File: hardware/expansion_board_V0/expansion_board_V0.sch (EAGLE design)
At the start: 502 parts, among them CON1 ELEC, CON10 M5, CON11 M2, CON12 M4, CON13 M1, CON14 ESC0, CON15 CON10_2_2.54, CON16 CON10_2_2.54, CON17 ESC1, CON18 UART0, CON19 QEI1, CON2 SERVO, CON20 AN0, CON21 S0, CON22 IO0, CON23 AN1, CON24 S1, CON25 IO1, CON26 UART1, CON27 QEI0, CON28 AN2, CON29 S2, CON3 LIPO_MOT, CON30 IO2, CON31 TELEM, CON32 QEI3, CON33 AN3, CON34 S3, CON35 IO3, CON36 BALISE, CON37 AN4, CON38 S4, CON39 IO4, CON4 LIPO_MOT, CON40 SPI0, CON41 QEI2, CON42 AN5, CON43 S5, CON44 IO5, CON45 SPI1, CON46 AN6, CON47 S6, CON48 IO6, CON49 I2C0, CON5 LIPO_MOT, CON50 AN7, CON51 S7, CON52 IO7, CON53 I2C1, CON54 USB2, CON55 USB3, CON56 USBfpga, CON57 FPGA_GPIO0, CON58 FPGA_GPIO1, CON59 FPGA_LTC, CON6 LIPO_MOT, CON60 USB3, CON61 CON5_2.54S, CON62 CON5_2.54S, CON63 CON5_2.54S, CON64 CON5_2.54S, CON7 FPGApower, CON8 M0, CON9 M3, IC1 ADS1258, IC2 ADS1278, IC3 REF5030I, IC4 REF5025I, J1 NC, J10 0, J11 0, J12 0, J13 0, J14 0, J15 0, J16 0, J17 0, J18 0, J19 0, J2 nc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

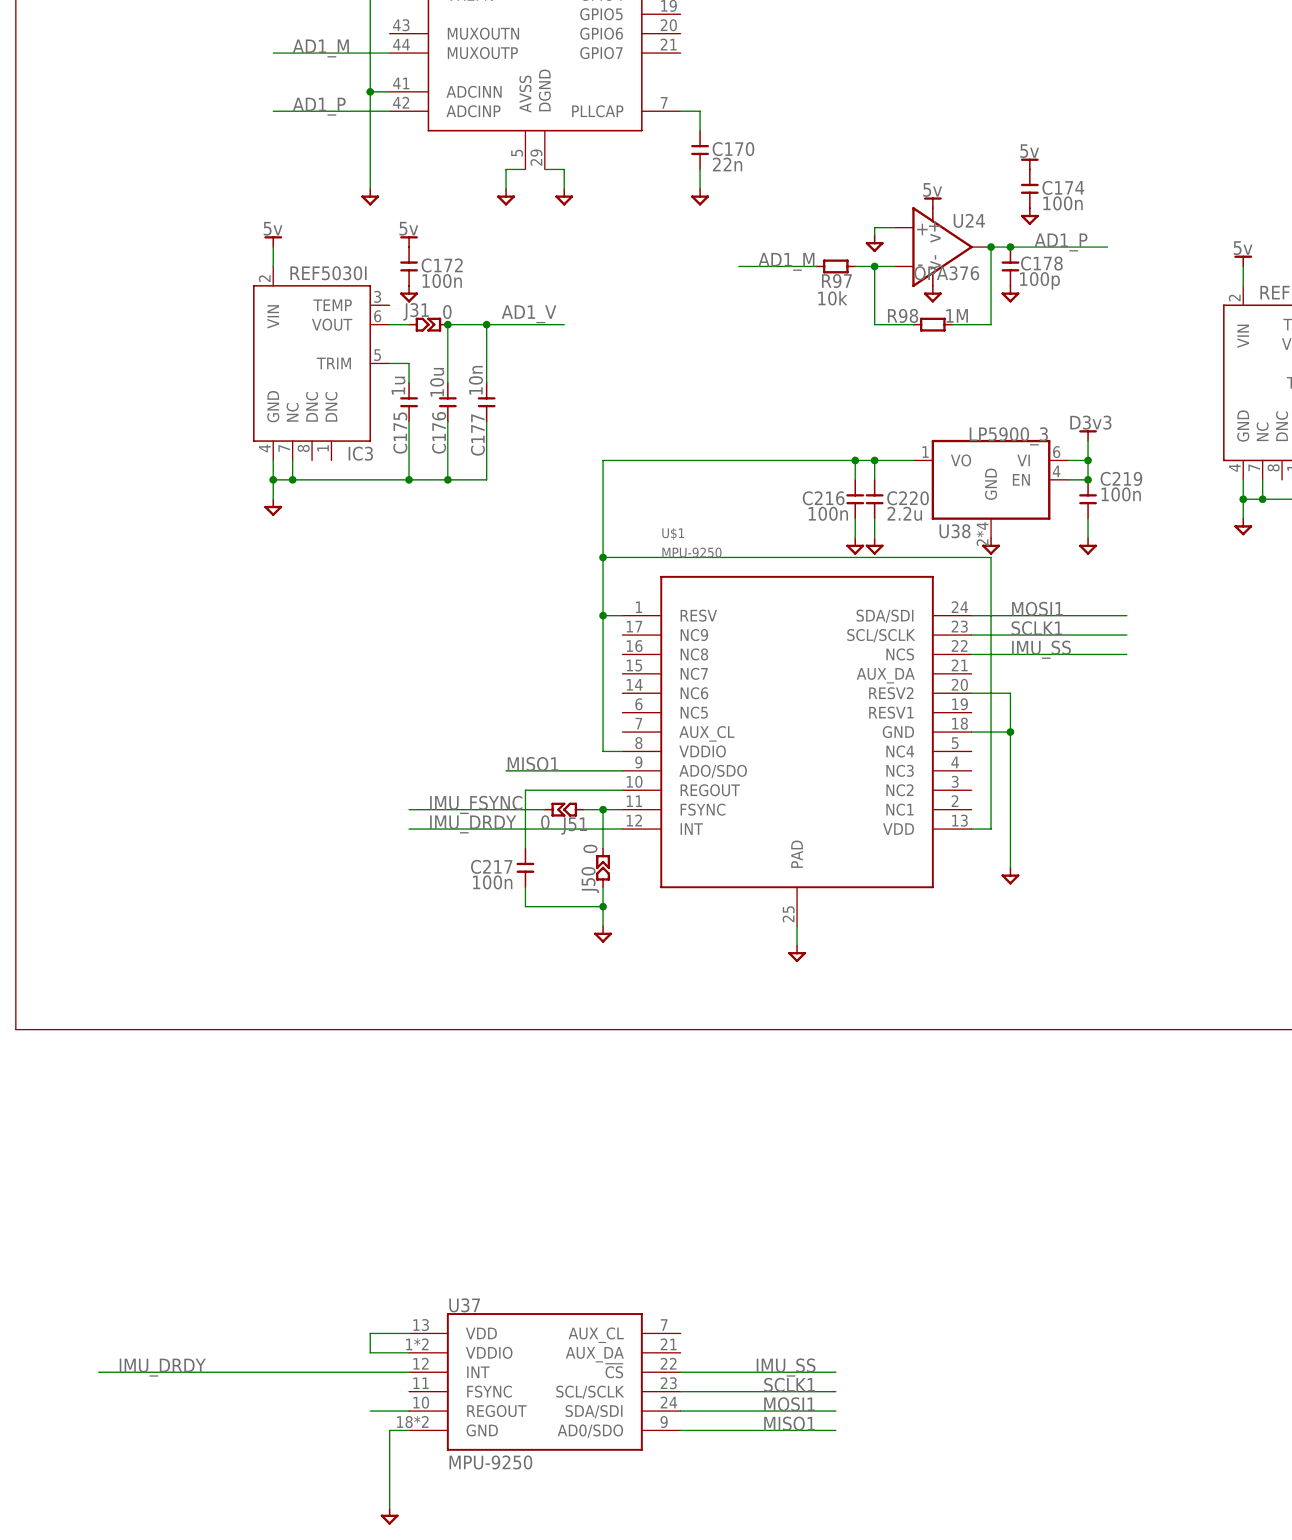
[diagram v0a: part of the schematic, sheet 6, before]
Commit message: IMU footprint ok Elec posté sur Eurocircuit
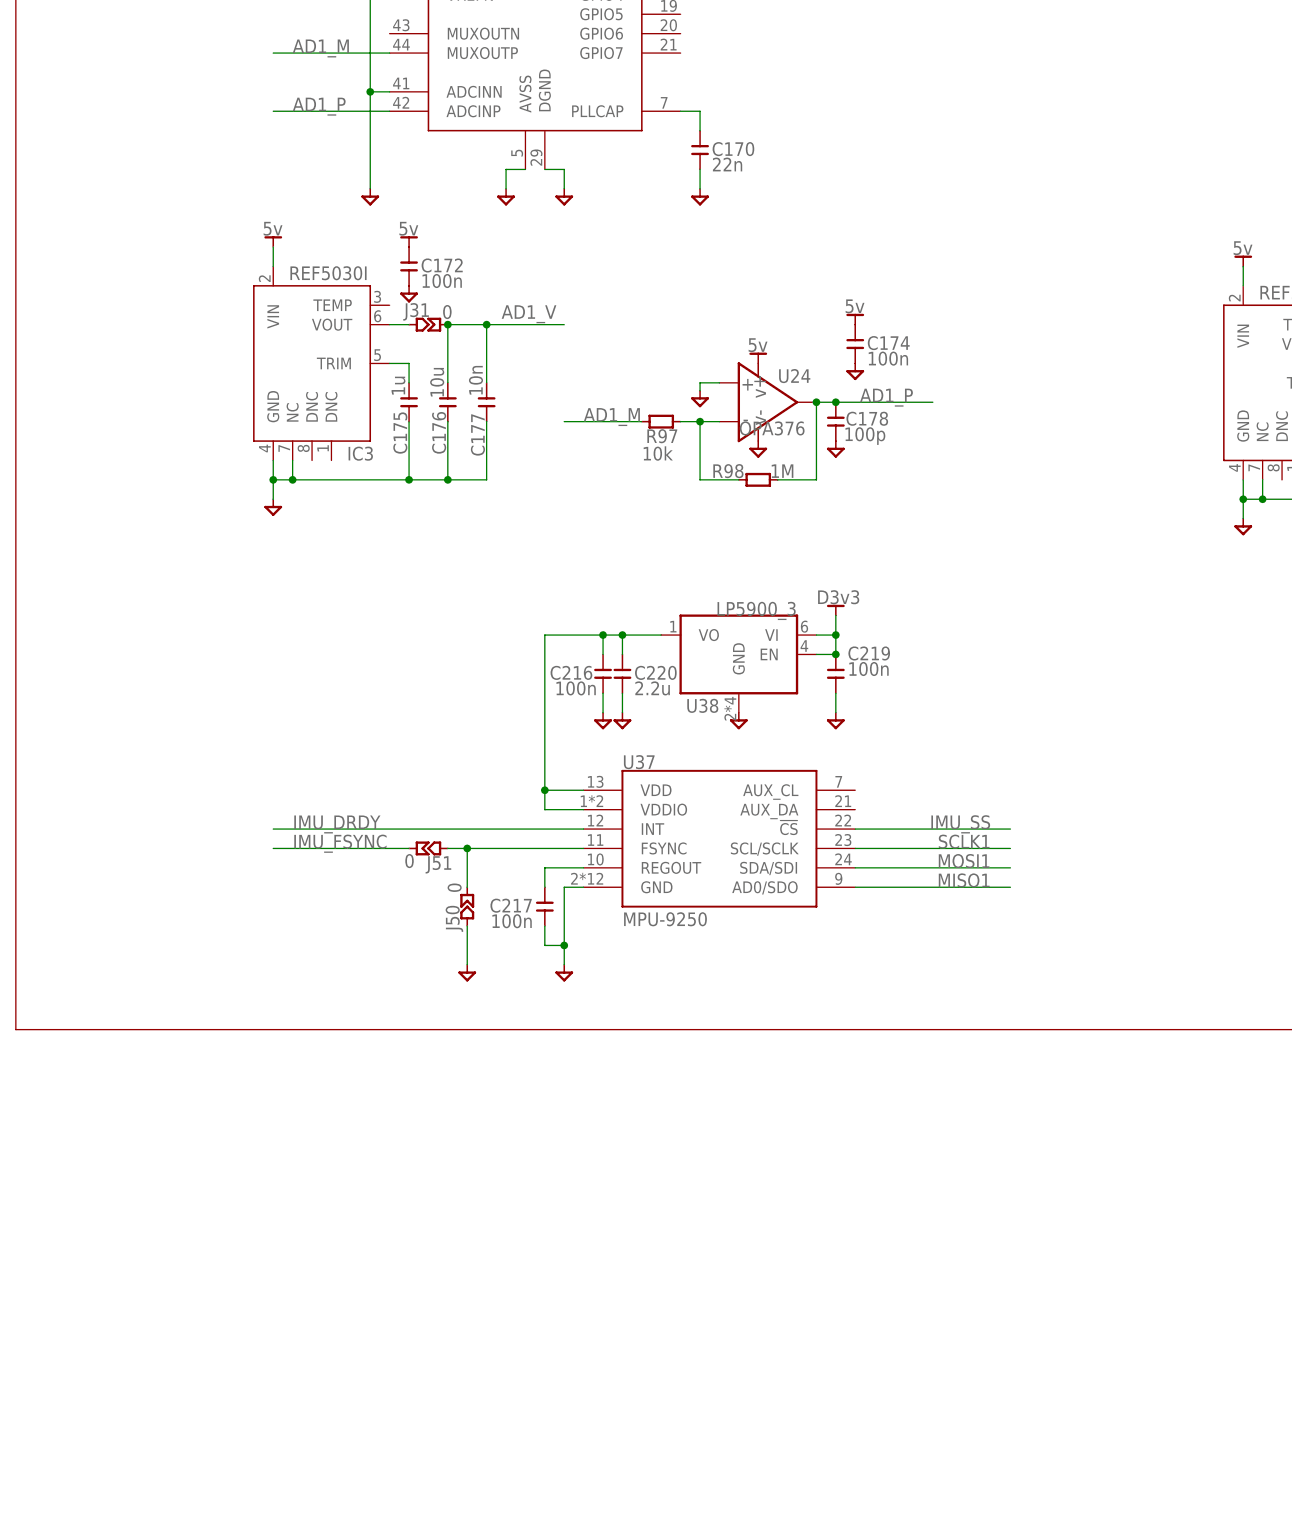
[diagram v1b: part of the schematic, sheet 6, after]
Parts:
- removed U$1: MPU-9250, invensense:MPU-9250
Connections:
- removed net N$107: C217.P$2, U$1.REGOUT
- removed net N$141: U37.VDD, U37.VDDIO
- net GND: no longer U$1.GND, U$1.PAD, U$1.RESV2
- net IMU_DRDY: no longer U$1.INT
- net IMU_SS: no longer U$1.NCS
- net MISO1: no longer U$1.ADO/SDO
- net MOSI1: no longer U$1.SDA/SDI
- net N$74: now also U37.VDD, U37.VDDIO; no longer U$1.RESV, U$1.VDD, U$1.VDDIO
- net N$98: now also U37.FSYNC; no longer U$1.FSYNC
- net REGOUT1: now also C217.P$2
- net SCLK1: no longer U$1.SCL/SCLK
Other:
- moved on the sheet: C174, C178, C216, C217, C219, C220, J50, J51, R97, R98, U24, U37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
